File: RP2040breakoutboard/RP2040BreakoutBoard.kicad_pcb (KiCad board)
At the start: 2 copper layers, 50 x 70 mm, 36 parts, among them J1 Conn_02x18_Odd_Even, J2 Conn_02x18_Odd_Even, J3 USB_C_Receptacle_USB2.0_14P, J4 Conn_01x02, U1 RP2040, U2 NCP1117-3.3_SOT223, U3 W25Q128JVS, X1 ABM8-272-T3

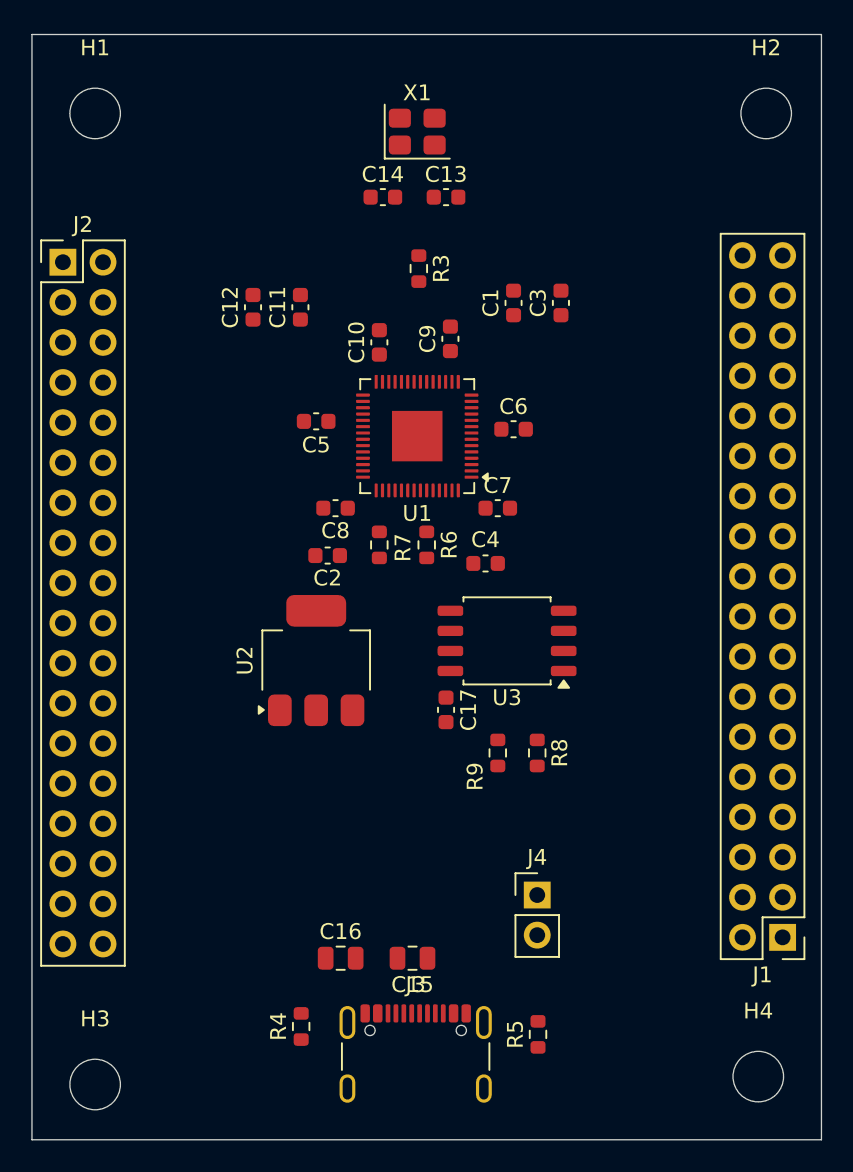
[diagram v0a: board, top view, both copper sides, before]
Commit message: Routed
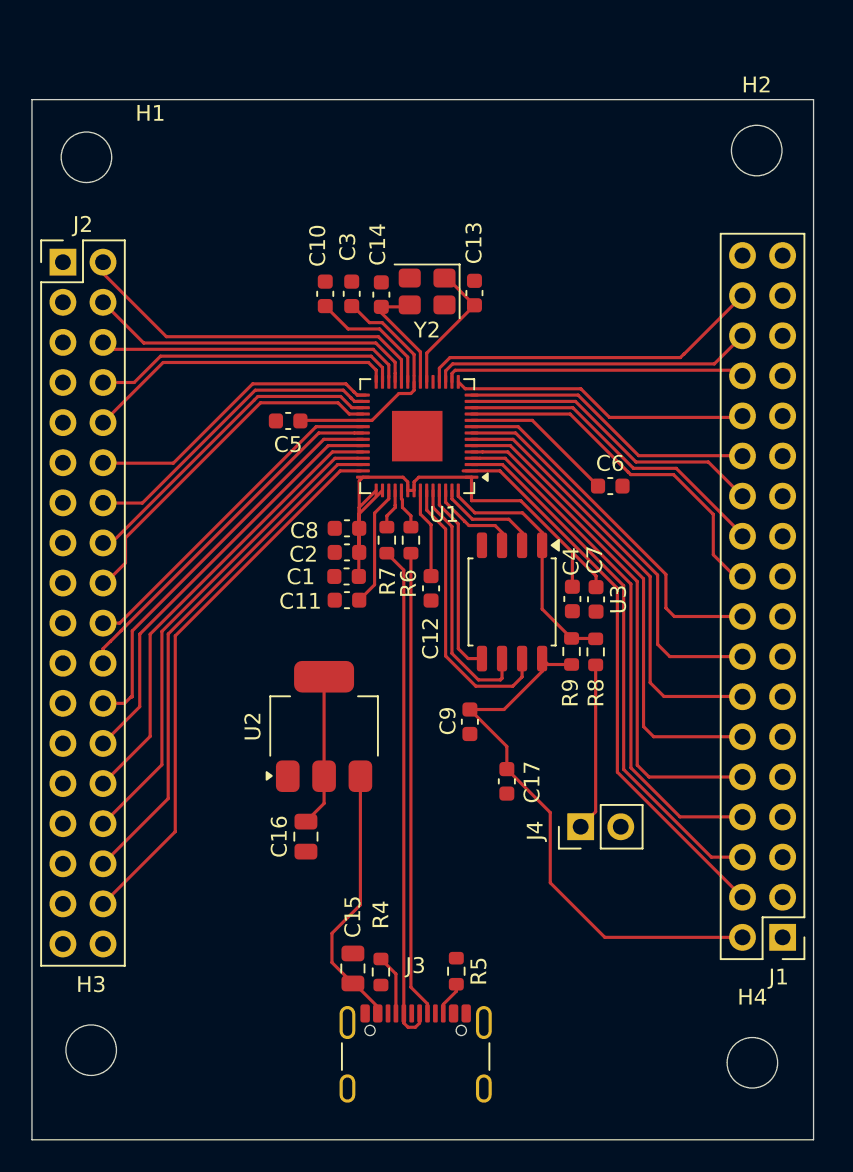
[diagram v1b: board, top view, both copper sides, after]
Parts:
- removed R3: 1k, Resistor_SMD:R_0603_1608Metric
- removed X1: ABM8-272-T3, Crystal:Crystal_SMD_3225-4Pin_3.2x2.5mm
- added Y2: Crystal_GND24, Crystal:Crystal_SMD_3225-4Pin_3.2x2.5mm, F.Cu at (93.5, 75.3)
- moved C9 24.3 mm to (96.2, 102.5), turned to -90 degrees
- moved C12 21.1 mm to (93.8, 94.1), turned to -90 degrees
- moved C1 20.3 mm to (88.4, 93.3), turned to 180 degrees
- moved C11 18.8 mm to (88.5, 94.8), turned to 180 degrees
- moved C3 13.3 mm to (88.8, 75.4)
- moved C7 8.49 mm to (104.2, 94.8), turned to -90 degrees
- moved C16 8.01 mm to (85.8, 109.8), turned to 90 degrees
- moved R9 7.95 mm to (102.7, 98.1)
- moved R8 7.39 mm to (104.2, 98.1)
- moved C6 7.10 mm to (105.1, 87.6)
- moved R5 6.54 mm to (95.4, 118.3), turned to -90 degrees
- moved C13 6.34 mm to (96.5, 75.4), turned to -90 degrees
- moved C14 6.18 mm to (90.6, 75.5), turned to 90 degrees
- moved R4 6.12 mm to (90.6, 118.4)
- moved C4 5.94 mm to (102.7, 94.8), turned to -90 degrees
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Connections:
- net /USB_DM renamed /USB_N
- net /USB_DP renamed /USB_P
- C11 pad 2: Net-(C11-Pad2) -> GND
- C12 pad 2: Net-(C11-Pad2) -> GND
- C13 pad 2: GND -> /XIN
- C14 pad 1: GND -> /XOUT
- J2 pad 2: /RUN -> /SWCLK
- J2 pad 6: /SWCLK -> /RUN
- U1 pad 20: GND -> /XIN
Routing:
- net +3V3: track 0.00 -> 105.8 mm
- net /GPIO0: track 0.00 -> 35.7 mm
- net /GPIO29: track 0.00 -> 34.9 mm
- net /GPIO1: track 0.00 -> 34.3 mm
- net /GPIO2: track 0.00 -> 33.4 mm
- net /GPIO28: track 0.00 -> 33.0 mm
- net /GPIO3: track 0.00 -> 32.5 mm
- net Net-(J3-D--PadA7): track 0.00 -> 32.0 mm
- net /GPIO27: track 0.00 -> 30.7 mm
- net /GPIO4: track 0.00 -> 30.3 mm
- net Net-(J3-D+-PadA6): track 0.00 -> 29.6 mm
- net /GPIO26: track 0.00 -> 29.0 mm
- net /GPIO5: track 0.00 -> 27.9 mm
- net /GPIO25: track 0.00 -> 27.0 mm
- net /GPIO24: track 0.00 -> 25.8 mm
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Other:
- board size 50 x 70 mm -> 49.5 x 65.9 mm
